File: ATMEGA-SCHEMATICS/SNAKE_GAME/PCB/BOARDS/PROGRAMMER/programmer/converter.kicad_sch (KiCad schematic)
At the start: 16 parts, among them J3 USB_A, SW5 SW_Push, U5 FT232RL

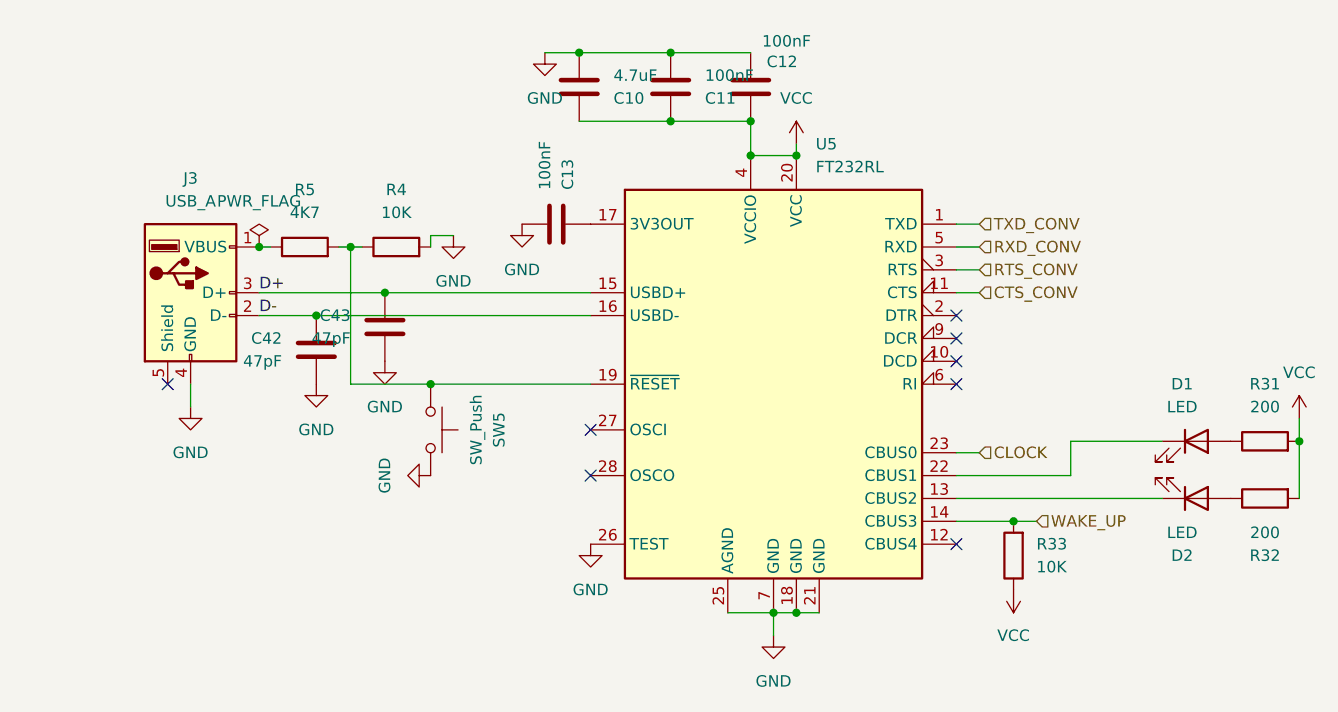
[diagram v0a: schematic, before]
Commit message: .
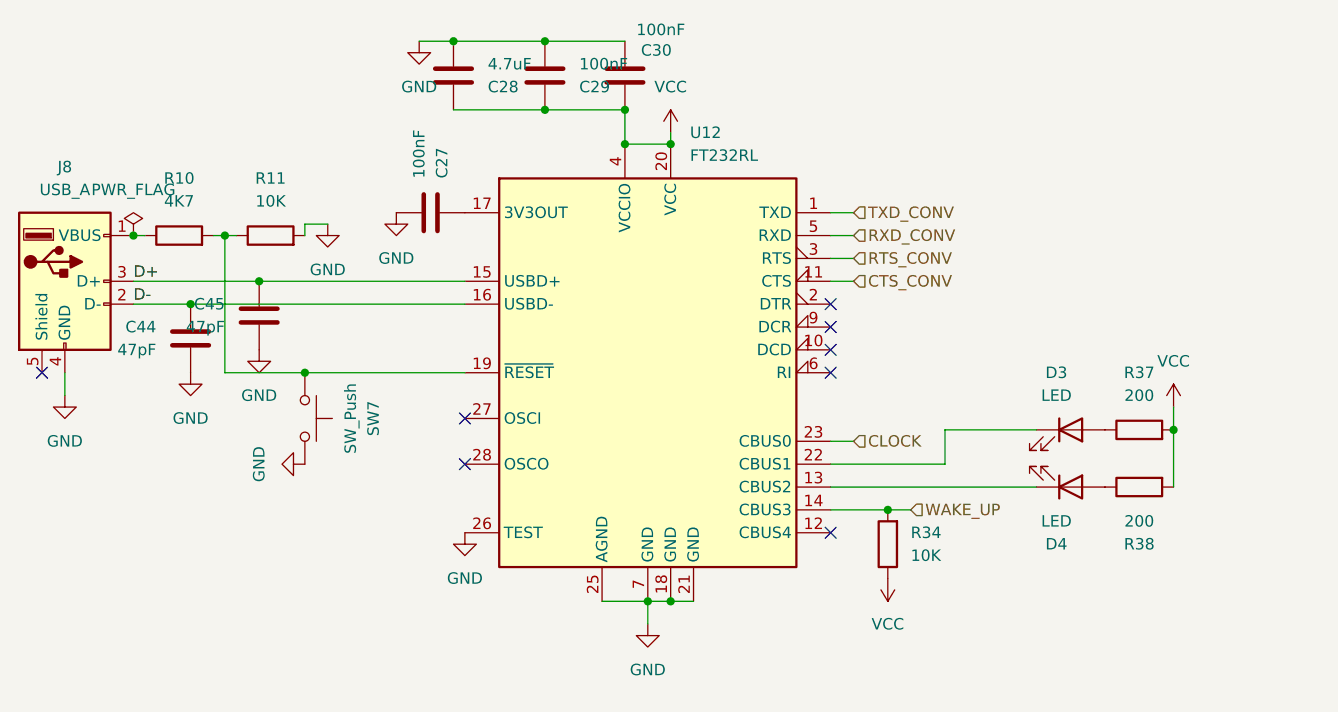
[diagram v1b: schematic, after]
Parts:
- removed C10: 4.7uF, Capacitor_THT:C_Disc_D7.5mm_W5.0mm_P5.00mm, symbol Device:C
- removed C11, C12, C13: 100nF, Capacitor_THT:C_Disc_D7.5mm_W5.0mm_P5.00mm, symbol Device:C
- removed C42, C43: 47pF, Capacitor_THT:C_Disc_D7.5mm_W5.0mm_P5.00mm, symbol Device:C
- removed D1, D2: LED, LED_THT:LED_D1.8mm_W3.3mm_H2.4mm, symbol Device:LED
- removed J3: USB_A, Connector_USB:USB_B_Lumberg_2411_02_Horizontal, symbol Connector:USB_A
- removed R31, R32: 200, Resistor_THT:R_Axial_DIN0207_L6.3mm_D2.5mm_P10.16mm_Horizontal, symbol Device:R
- removed R33, R4: 10K, Resistor_THT:R_Axial_DIN0207_L6.3mm_D2.5mm_P10.16mm_Horizontal, symbol Device:R
- removed R5: 4K7, Resistor_THT:R_Axial_DIN0207_L6.3mm_D2.5mm_P10.16mm_Horizontal, symbol Device:R
- removed SW5: SW_Push, Button_Switch_THT:SW_PUSH_1P1T_6x3.5mm_H4.3_APEM_MJTP1243, symbol Switch:SW_Push
- removed U5: FT232RL, Package_DIP:DIP-28_W15.24mm_LongPads, symbol Interface_USB:FT232RL
- added C27, C29, C30: 100nF, Capacitor_SMD:C_0402_1005Metric, symbol Device:C
- added C28: 4.7uF, Capacitor_SMD:C_0805_2012Metric, symbol Device:C
- added C44, C45: 47pF, Capacitor_THT:C_Disc_D7.5mm_W5.0mm_P5.00mm, symbol Device:C
- added D3, D4: LED, LED_THT:LED_D1.8mm_W3.3mm_H2.4mm, symbol Device:LED
- added J8: USB_A, Connector_USB:USB_B_Lumberg_2411_02_Horizontal, symbol Connector:USB_A
- added R10: 4K7, Resistor_THT:R_Axial_DIN0207_L6.3mm_D2.5mm_P10.16mm_Horizontal, symbol Device:R
- added R11, R34: 10K, Resistor_THT:R_Axial_DIN0207_L6.3mm_D2.5mm_P10.16mm_Horizontal, symbol Device:R
- added R37, R38: 200, Resistor_THT:R_Axial_DIN0207_L6.3mm_D2.5mm_P10.16mm_Horizontal, symbol Device:R
- added SW7: SW_Push, Button_Switch_THT:SW_PUSH_1P1T_6x3.5mm_H4.3_APEM_MJTP1243, symbol Switch:SW_Push
- added U12: FT232RL, Package_DIP:DIP-28_W15.24mm_LongPads, symbol Interface_USB:FT232RL
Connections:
- net CLOCK: now also U12.23 (CBUS0)
- net CTS_CONV: now also U12.11 (CTS)
- net D+: now also C45.1, J8.3 (D+), U12.15 (USBD+)
- net D-: now also C44.1, J8.2 (D-), U12.16 (USBD-)
- net GND: now also C27.2, C28.2, C29.2, C30.2, C44.2, C45.2, J8.4 (GND), R11.2, SW7.2, U12.18 (GND), U12.21 (GND), U12.25 (AGND), U12.26 (TEST), U12.7 (GND)
- net RTS_CONV: now also U12.3 (RTS)
- net RXD_CONV: now also U12.5 (RXD)
- net TXD_CONV: now also U12.1 (TXD)
- net VCC: now also C28.1, C29.1, C30.1, R34.1, R37.2, R38.2, U12.20 (VCC), U12.4 (VCCIO)
- net WAKE_UP: now also R34.2, U12.14 (CBUS3)
- new net: R10.2, R11.1, SW7.1, U12.19 (~{RESET})
- new net: J8.1 (VBUS), R10.1
- new net: D4.1 (K), U12.13 (CBUS2)
- new net: D4.2 (A), R38.1
- new net: D3.2 (A), R37.1
- new net: D3.1 (K), U12.22 (CBUS1)
- new net: C27.1, U12.17 (3V3OUT)
